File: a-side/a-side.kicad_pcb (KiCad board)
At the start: 2 copper layers, 100 x 70 mm, 56 parts, among them IC3 GL823K, IC4 GL823K, J1 USB_A, J2 SD_Card_Receptacle, J3 USB_A, J4 USB_C_Receptacle_USB2.0_14P, J5 SD_Card_Receptacle, SW1 SW_Push, U1 SRV05-4, U2 SRV05-4, Y1 12MHz

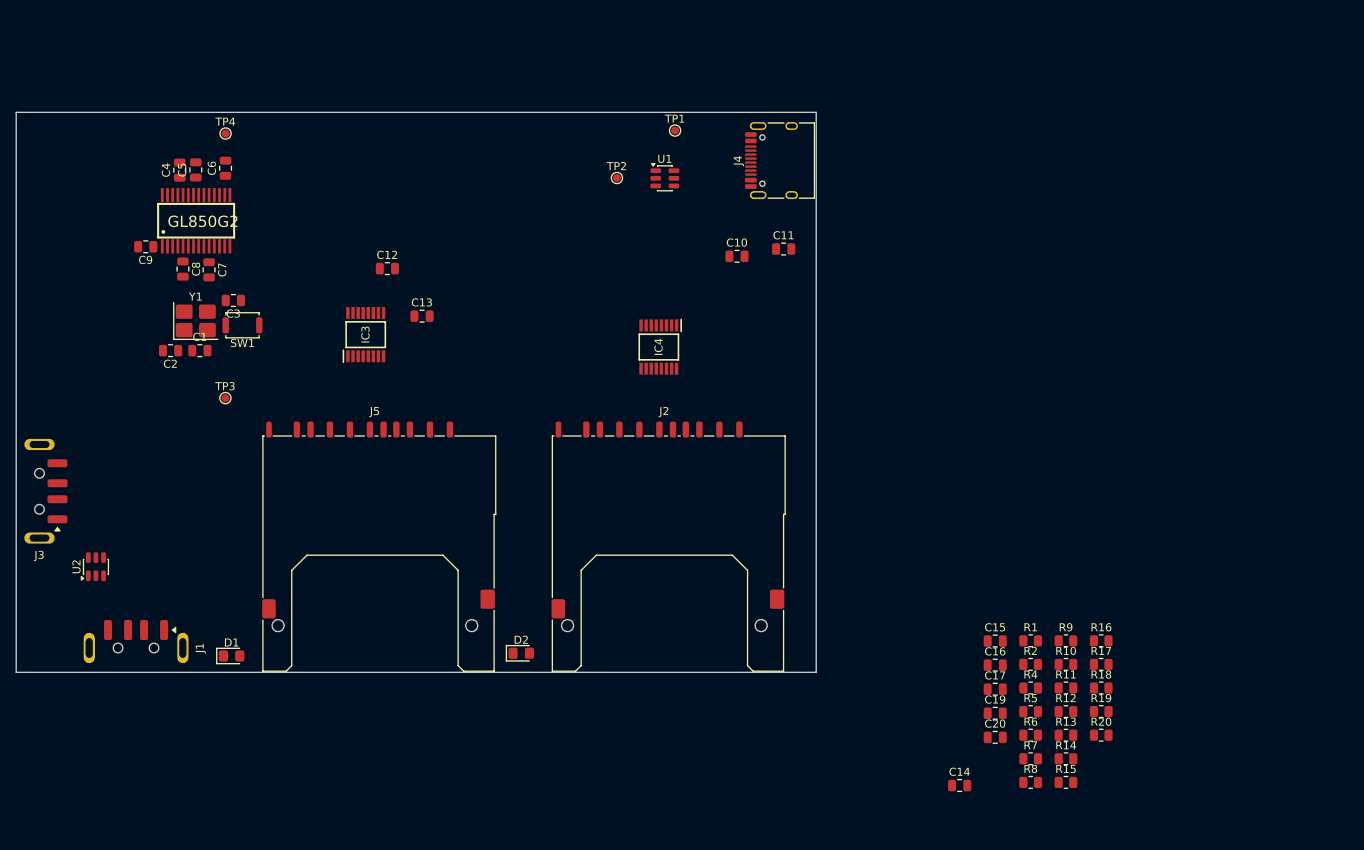
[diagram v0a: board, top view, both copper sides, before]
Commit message: DOME
done done done DONE 0 errors 108982 warnings who gaf im done
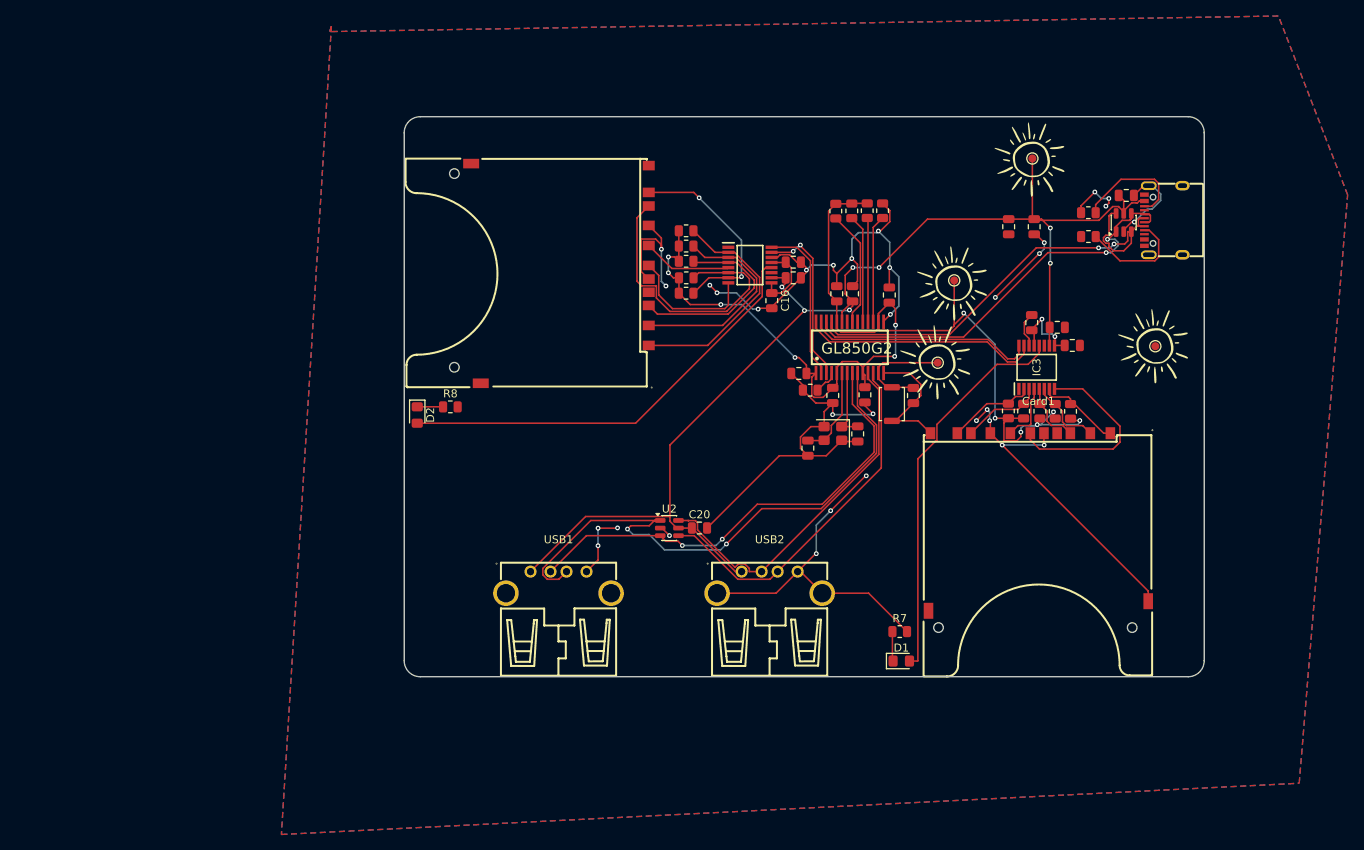
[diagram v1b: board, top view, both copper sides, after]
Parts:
- removed J1, J3: USB_A, Connector_USB:USB_A_Connfly_DS1098_Horizontal
- removed J2, J5: SD_Card_Receptacle, Connector_Card:SD_Kyocera_145638009511859+
- removed J4: USB_C_Receptacle_USB2.0_14P, Connector_USB:USB_C_Receptacle_HRO_TYPE-C-31-M-12
- removed R9: 5.1k, Resistor_SMD:R_0805_2012Metric
- removed Y1: 12MHz, Crystal:Crystal_SMD_3225-4Pin_3.2x2.5mm_HandSoldering
- added Card1: SD-106M, easyeda2kicad:SD-SMD_SD-106M, F.Cu at (178.5, 101.0)
- added Card2: SD-106M, easyeda2kicad:SD-SMD_SD-106M, F.Cu at (118.7, 70.0)
- added G***: LOGO, LOGO, F.Cu at (165.8, 80.9)
- added G***: LOGO, LOGO, B.Cu at (132.8, 90.9)
- added G***: LOGO, LOGO, B.Cu at (158.6, 71.7)
- added G***: LOGO, LOGO, F.Cu at (167.9, 71.0)
- added G***: LOGO, LOGO, F.Cu at (193.1, 78.9)
- added G***: LOGO, LOGO, F.Cu at (177.6, 55.5)
- added G***: LOGO, LOGO, B.Cu at (179.4, 100.2)
- added G***: LOGO, LOGO, B.Cu at (130.6, 71.4)
- added G***: LOGO, LOGO, B.Cu at (105.1, 85.2)
- added G***: LOGO, LOGO, B.Cu at (133.0, 111.5)
- added G***: LOGO, LOGO, B.Cu at (187.2, 69.5)
- added R23: 5.1k, Resistor_SMD:R_0805_2012Metric, F.Cu at (184.7, 65.4)
- added USB1: AF 90° WJDG, easyeda2kicad:USB-A-TH_AF-WJDG, F.Cu at (118.5, 108.6)
- added USB2: AF 90° WJDG, easyeda2kicad:USB-A-TH_AF-WJDG, F.Cu at (144.9, 108.6)
- added USB3: TYPE-C 16PIN 2MD, easyeda2kicad:USB-C-SMD_TYPE-C-16PIN-2MD-073, F.Cu at (194.1, 63.3)
- added Y2: Crystal_GND24, Crystal:Crystal_SMD_3225-4Pin_3.2x2.5mm, F.Cu at (152.8, 90.0)
- moved TP4 92.9 mm to (168.0, 70.8)
- moved TP3 89.1 mm to (165.9, 81.1)
- moved C2 86.5 mm to (155.9, 90.0), turned to -90 degrees
- moved R8 86.4 mm to (105.0, 86.7)
- moved C12 86.2 mm to (182.7, 79.0)
- moved C3 85.8 mm to (162.9, 85.2), turned to 90 degrees
- moved C6 84.5 mm to (159.9, 72.7)
- moved IC3 84.0 mm to (178.3, 81.7)
- moved D1 83.7 mm to (161.4, 118.4)
- moved C4 83.6 mm to (153.3, 72.5)
- moved C5 83.5 mm to (155.3, 72.5)
- moved C7 83.5 mm to (156.8, 85.1)
- moved GL850G2 83.2 mm to (154.9, 79.2)
- moved C9 83.2 mm to (148.6, 82.5)
- moved C8 82.8 mm to (152.8, 85.2)
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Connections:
- IC3 pad 10: GND -> VBUS
- IC4 pad 10: GND -> VBUS
- R11 pad 1: +3V3 -> +3.3V
- R12 pad 1: +3V3 -> +3.3V
- R13 pad 1: +3V3 -> +3.3V
- R14 pad 1: +3V3 -> +3.3V
- R15 pad 1: +3V3 -> +3.3V
- R16 pad 1: +3V3 -> +3.3V
- R17 pad 1: +3V3 -> +3.3V
- R18 pad 1: +3V3 -> +3.3V
- R19 pad 1: +3V3 -> +3.3V
- R2 pad 2: +3V3 -> +3.3V
- R20 pad 1: +3V3 -> +3.3V
- R5 pad 2: +3V3 -> +3.3V
- R6 pad 2: +3V3 -> +3.3V
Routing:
- net GND: track 0.00 -> 271.5 mm, vias 0 -> 32
- net VBUS: track 0.00 -> 155.9 mm, vias 0 -> 7
- net +3.3V: track 0.00 -> 146.7 mm, vias 0 -> 12
- net /USBA1_DP: track 0.00 -> 74.3 mm, vias 0 -> 2
- net /USB_DM: track 0.00 -> 59.6 mm, vias 0 -> 2
- net /USBA1_DM: track 0.00 -> 58.7 mm, vias 0 -> 2
- net Net-(D2-A): track 0.00 -> 54.2 mm
- net /USB_DP: track 0.00 -> 53.4 mm, vias 0 -> 2
- net Net-(D1-A): track 0.00 -> 49.1 mm
- net /USBA2_DP: track 0.00 -> 45.7 mm
- net /USBA2_DM: track 0.00 -> 45.6 mm
- net /SD2_D0: track 0.00 -> 36.5 mm
- net /SD1_DP: track 0.00 -> 30.0 mm
- net /SD2_D2: track 0.00 -> 29.2 mm
- net /SD1_DM: track 0.00 -> 28.4 mm
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- added copper zone on B.Cu, net GND
- added copper zone on F.Cu, net GND
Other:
- outline, holes or cut-outs redrawn
- board text added: "made with music and <3 by sua"
